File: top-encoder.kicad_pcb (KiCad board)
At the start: 2 copper layers, 8 parts, among them M1 THRU_HOLE_PAD, M2 THRU_HOLE_PAD, M3 THRU_HOLE_PAD, M4 THRU_HOLE_PAD, U2 TLE5009E1000FUMA1

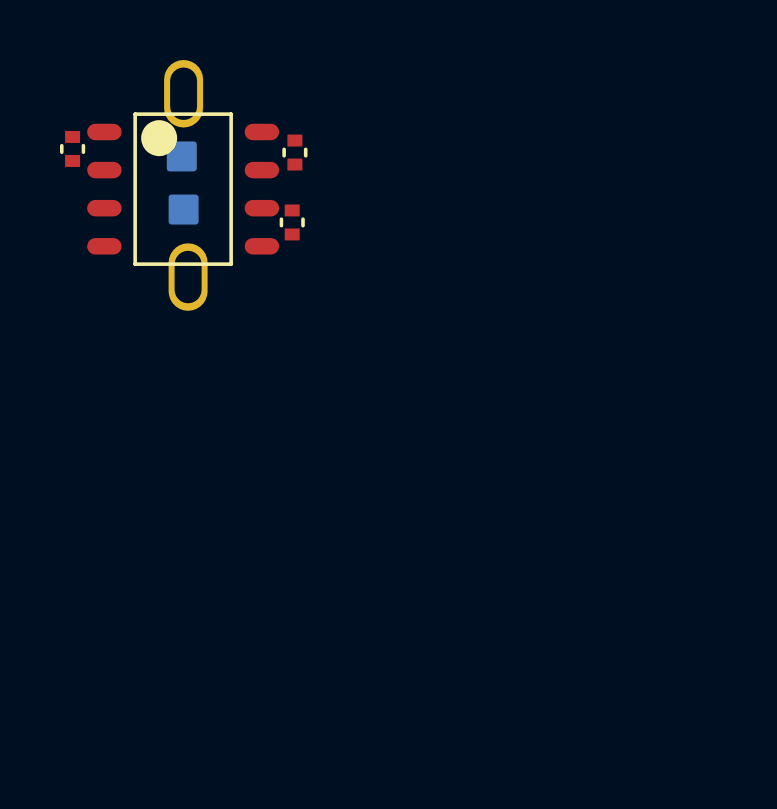
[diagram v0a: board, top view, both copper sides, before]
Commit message: designed dogbone
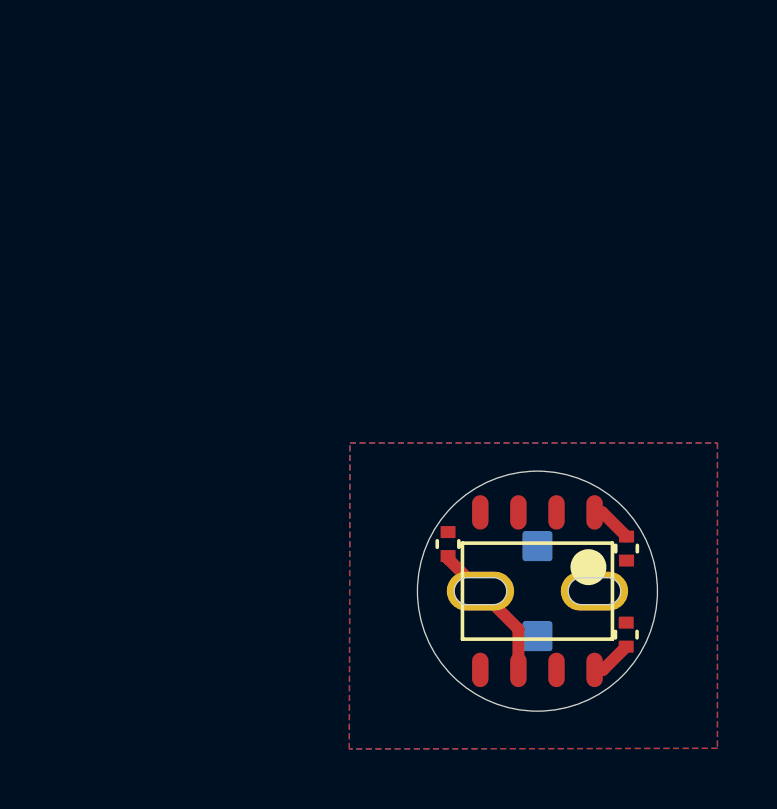
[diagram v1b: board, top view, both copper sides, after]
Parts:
- moved C2 22.8 mm to (145.0, 93.8)
- moved M4 21.5 mm to (143.9, 95.2), turned to 180 degrees
- moved C3 19.5 mm to (145.0, 96.7), turned to 90 degrees
- moved M3 18.5 mm to (142.0, 96.8), turned to -90 degrees
- moved U2 17.9 mm to (142.0, 95.2), turned to -90 degrees
- moved M2 17.6 mm to (142.0, 93.8), turned to -90 degrees
- moved M1 14.3 mm to (140.1, 95.2), turned to 180 degrees
- moved C1 11.9 mm to (139.1, 93.7), turned to 90 degrees
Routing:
- net /3v3: track 0.00 -> 4.77 mm
- net /COS: track 0.00 -> 1.40 mm
- net /SIN: track 0.00 -> 1.38 mm
- added copper zone on B.Cu, net GND
- added copper zone on F.Cu, net GND
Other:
- board outline added: 8 x 8 mm
